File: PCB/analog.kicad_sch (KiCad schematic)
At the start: 13 parts, among them U3 74HC4051, U4 OPA350

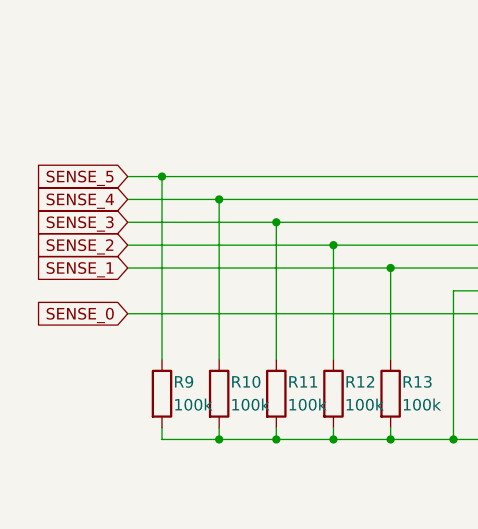
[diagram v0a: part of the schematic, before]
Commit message: WIP PCB
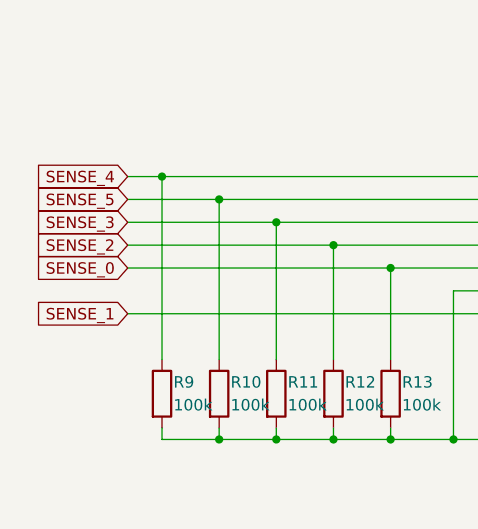
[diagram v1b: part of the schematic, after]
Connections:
- net SENSE_0: now also R13.1, U3.1 (A4); no longer R14.1, U3.2 (A6)
- net SENSE_1: now also R14.1, U3.2 (A6); no longer R13.1, U3.1 (A4)
- net SENSE_4: now also R9.1, U3.13 (A0); no longer R10.1, U3.14 (A1)
- net SENSE_5: now also R10.1, U3.14 (A1); no longer R9.1, U3.13 (A0)
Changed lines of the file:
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@@
   (title_block
     (title "EC23U - Analog")
-    (date "2022-11-10")
+    (date "2022-11-11")
     (rev "1")
     (company "Cipulot PCB Design")
@@
     )
   )
-  (global_label "SENSE_1" (shape input) (at 24.765 41.275 180) (fields_autoplaced)
+  (global_label "SENSE_4" (shape input) (at 24.765 31.115 180) (fields_autoplaced)
+    (effects (font (size 1.27 1.27)) (justify right))
+    (property "Intersheet References" "${INTERSHEET_REFS}" (id 0) (at 14.1271 31.0356 0)
+      (effects (font (size 1.27 1.27)) (justify right) hide)
+    )
+  )
+  (global_label "SENSE_3" (shape input) (at 24.765 36.195 180) (fields_autoplaced)
+    (effects (font (size 1.27 1.27)) (justify right))
+    (property "Intersheet References" "${INTERSHEET_REFS}" (id 0) (at 14.1271 36.1156 0)
+      (effects (font (size 1.27 1.27)) (justify right) hide)
+    )
+  )
+  (global_label "AMUX_SEL_1" (shape input) (at 100.965 38.735 0) (fields_autoplaced)
+    (effects (font (size 1.27 1.27)) (justify left))
+    (property "Intersheet References" "${INTERSHEET_REFS}" (id 0) (at 114.9895 38.6556 0)
+      (effects (font (size 1.27 1.27)) (justify left) hide)
+    )
+  )
+  (global_label "SENSE_0" (shape input) (at 24.765 41.275 180) (fields_autoplaced)
     (effects (font (size 1.27 1.27)) (justify right))
     (property "Intersheet References" "${INTERSHEET_REFS}" (id 0) (at 14.1271 41.1956 0)
@@
     )
   )
-  (global_label "SENSE_5" (shape input) (at 24.765 31.115 180) (fields_autoplaced)
-    (effects (font (size 1.27 1.27)) (justify right))
-    (property "Intersheet References" "${INTERSHEET_REFS}" (id 0) (at 14.1271 31.0356 0)
-      (effects (font (size 1.27 1.27)) (justify right) hide)
-    )
-  )
-  (global_label "SENSE_3" (shape input) (at 24.765 36.195 180) (fields_autoplaced)
-    (effects (font (size 1.27 1.27)) (justify right))
-    (property "Intersheet References" "${INTERSHEET_REFS}" (id 0) (at 14.1271 36.1156 0)
-      (effects (font (size 1.27 1.27)) (justify right) hide)
-    )
-  )
-  (global_label "AMUX_SEL_1" (shape input) (at 100.965 38.735 0) (fields_autoplaced)
-    (effects (font (size 1.27 1.27)) (justify left))
-    (property "Intersheet References" "${INTERSHEET_REFS}" (id 0) (at 114.9895 38.6556 0)
-      (effects (font (size 1.27 1.27)) (justify left) hide)
+  (global_label "SENSE_1" (shape input) (at 24.765 46.355 180) (fields_autoplaced)
+    (effects (font (size 1.27 1.27)) (justify right))
+    (property "Intersheet References" "${INTERSHEET_REFS}" (id 0) (at 14.1271 46.2756 0)
+      (effects (font (size 1.27 1.27)) (justify right) hide)
     )
   )
@@
     )
   )
-  (global_label "SENSE_4" (shape input) (at 24.765 33.655 180) (fields_autoplaced)
+  (global_label "SENSE_5" (shape input) (at 24.765 33.655 180) (fields_autoplaced)
     (effects (font (size 1.27 1.27)) (justify right))
     (property "Intersheet References" "${INTERSHEET_REFS}" (id 0) (at 14.1271 33.5756 0)
       (effects (font (size 1.27 1.27)) (justify right) hide)
     )
-  )
-  (global_label "SENSE_0" (shape input) (at 24.765 46.355 180) (fields_autoplaced)
-    (effects (font (size 1.27 1.27)) (justify right))
-    (property "Intersheet References" "${INTERSHEET_REFS}" (id 0) (at 14.1271 46.2756 0)
-      (effects (font (size 1.27 1.27)) (justify right) hide)
-    )
